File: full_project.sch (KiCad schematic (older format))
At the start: 42 parts, among them J1 Conn_01x16, J12 V_OFFSET, J14 Conn_01x02, J2 Raspberry_Pi_2_3, J3 Conn_01x08, J4 Screw_Terminal_01x04_titrator, J5 RF_Shield_Two_Pieces, J6 BNC_Jack, J7 SJ-43515TS, J8 Screw_Terminal_01x03, J9 SJ-43515TS, Q1 PN2222A, U1 ADS1115_BO, U2 A4988_BO, U3 MAX31865_BO, U4 MAX31865_BO, U5 LT1634, U6 LMC662, U7 LMC662, U8 L7805

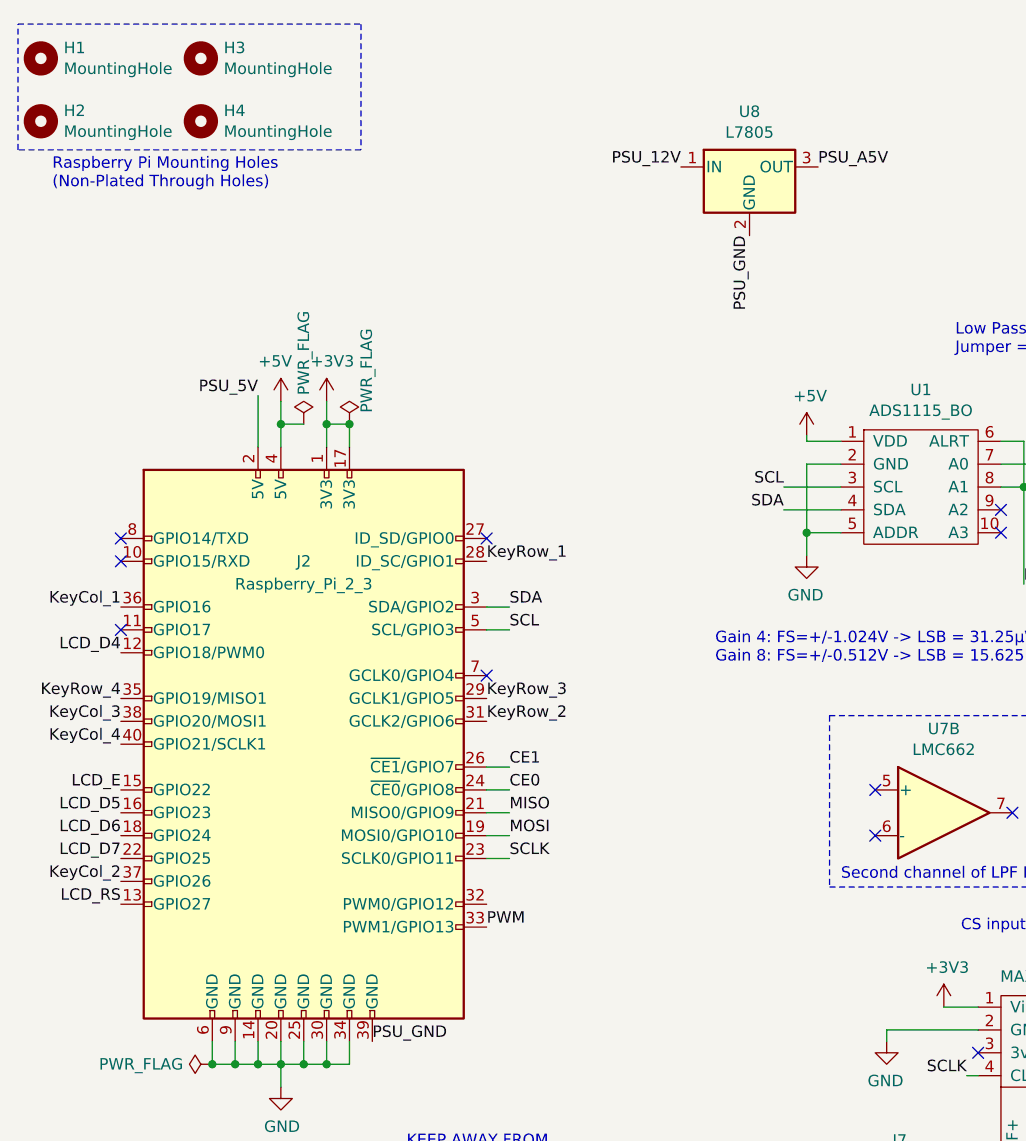
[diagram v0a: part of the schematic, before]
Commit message: not much
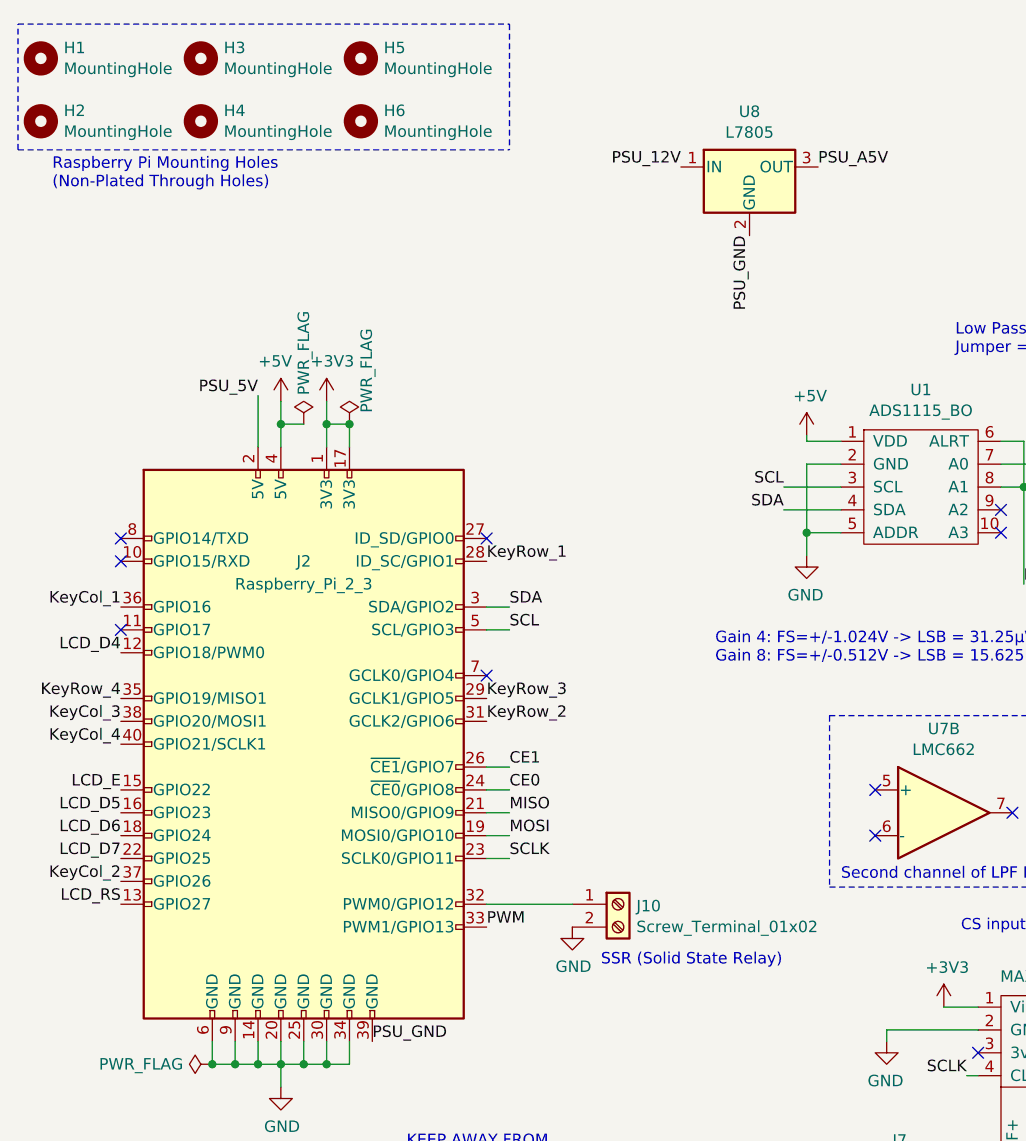
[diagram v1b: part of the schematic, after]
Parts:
- added H5, H6: MountingHole, MountingHole:MountingHole_3mm, symbol Mechanical:MountingHole
- added J10: Screw_Terminal_01x02, TerminalBlock:TerminalBlock_bornier-2_P5.08mm, symbol Connector:Screw_Terminal_01x02
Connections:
- net GND: now also J10.2 (Pin_2)
- net at J2.32 (PWM0/GPIO12): now also J10.1 (Pin_1)
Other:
- note added: "SSR (Solid State Relay)"
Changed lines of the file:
@@
 $EndComp
 Wire Notes Line
-	550  550  2050 550
-Wire Notes Line
-	2050 550  2050 1100
-Wire Notes Line
-	2050 1100 550  1100
+	2700 550  2700 1100
 Wire Notes Line
 	550  1100 550  550
@@
 	1    0    0    -1
 $EndComp
+$Comp
+L Mechanical:MountingHole H5
+U 1 1 604871C9
+P 2050 700
+F 0 "H5" H 2150 746 50  0000 L CNN
+F 1 "MountingHole" H 2150 655 50  0000 L CNN
+F 2 "MountingHole:MountingHole_3mm" H 2050 700 50  0001 C CNN
+F 3 "~" H 2050 700 50  0001 C CNN
+	1    2050 700
+	1    0    0    -1
+$EndComp
+$Comp
+L Mechanical:MountingHole H6
+U 1 1 60491872
+P 2050 975
+F 0 "H6" H 2150 1021 50  0000 L CNN
+F 1 "MountingHole" H 2150 930 50  0000 L CNN
+F 2 "MountingHole:MountingHole_3mm" H 2050 975 50  0001 C CNN
+F 3 "~" H 2050 975 50  0001 C CNN
+	1    2050 975
+	1    0    0    -1
+$EndComp
+Wire Notes Line
+	550  550  2700 550
+Wire Notes Line
+	550  1100 2700 1100
+$Comp
+L Connector:Screw_Terminal_01x02 J10
+U 1 1 604B33B0
+P 3175 4400
+F 0 "J10" H 3255 4392 50  0000 L CNN
+F 1 "Screw_Terminal_01x02" H 3255 4301 50  0000 L CNN
+F 2 "TerminalBlock:TerminalBlock_bornier-2_P5.08mm" H 3175 4400 50  0001 C CNN
+F 3 "~" H 3175 4400 50  0001 C CNN
+	1    3175 4400
+	1    0    0    -1
+$EndComp
+Wire Wire Line
+	2600 4400 2975 4400
+$Comp
+L power:GND #PWR016
+U 1 1 604C156D
+P 2975 4500
+F 0 "#PWR016" H 2975 4250 50  0001 C CNN
+F 1 "GND" H 2980 4327 50  0000 C CNN
+F 2 "" H 2975 4500 50  0001 C CNN
+F 3 "" H 2975 4500 50  0001 C CNN
+	1    2975 4500
+	1    0    0    -1
+$EndComp
+Text Notes 3100 4675 0    50   ~ 0
+SSR (Solid State Relay)
 $EndSCHEMATC
